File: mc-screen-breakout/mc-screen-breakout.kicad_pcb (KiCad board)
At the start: 4 copper layers, 32 x 20 mm, 28 parts, among them J1 USB_C_Receptacle_PowerOnly_6P, J2 FH28-10S-0.5SH_05_, SW1 NANOT160BP, SW2 NANOT160BP, U1 CMM-3424DT-26165-TR, U2 MDBT50Q-1MV2, Y1 32.768kHz

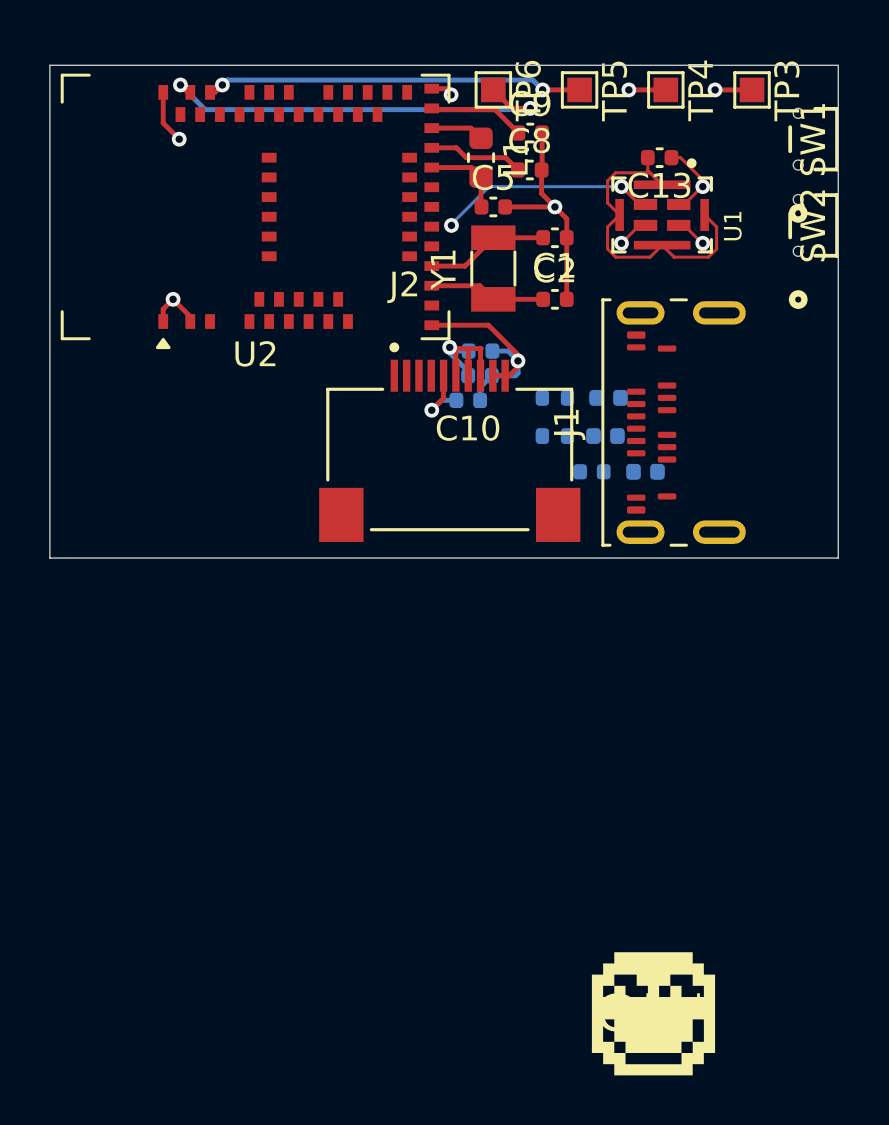
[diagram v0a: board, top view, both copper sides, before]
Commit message: More routing
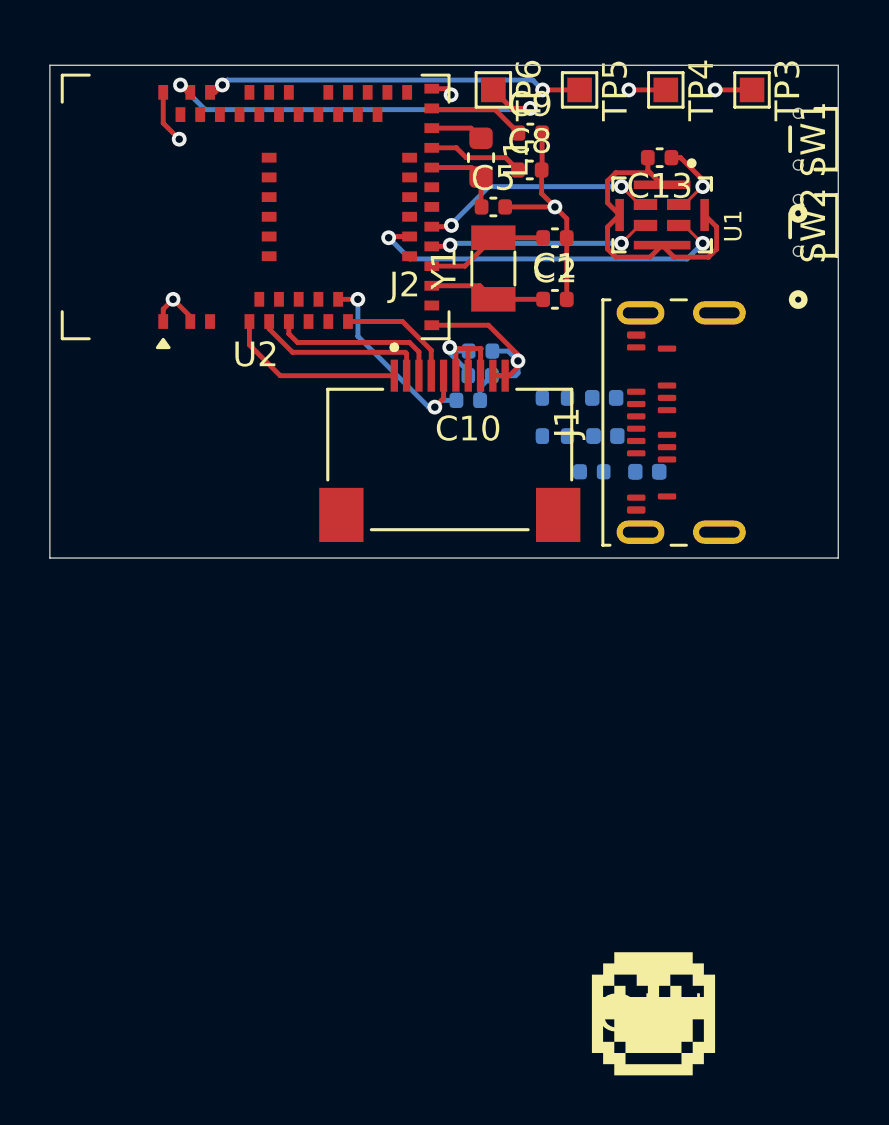
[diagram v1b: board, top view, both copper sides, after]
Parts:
- moved D2 0.17 mm to (58.0, 28.0)
- moved D3 0.08 mm to (59.8, 31.0)
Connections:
- C3 pad 1: +BATT -> Net-(D3-A1)
- D1 pad 2: Net-(D1-A2) -> GND
- D2 pad 2: Net-(D2-A2) -> GND
- D3 pad 2: +BATT -> GND
- R1 pad 1: Net-(D1-A2) -> Net-(D1-A1)
- R2 pad 2: Net-(D2-A2) -> Net-(D2-A1)
- U2 pad 13: unconnected-(U2-P0.28-Pad13) -> LCD_DISP
- U2 pad 14: unconnected-(U2-P0.30-Pad14) -> LCD_EXCOMIN
- U2 pad 16: LCD_DISP -> unconnected-(U2-P0.27-Pad16)
- U2 pad 19: LCD_EXCOMIN -> unconnected-(U2-P0.26-Pad19)
- U2 pad 20: unconnected-(U2-P0.04-Pad20) -> MIC_CLK
- U2 pad 21: unconnected-(U2-P0.05-Pad21) -> MIC_DATA
- U2 pad 22: unconnected-(U2-P0.06-Pad22) -> MIC_SELECT
- U2 pad 4: unconnected-(U2-P1.11-Pad4) -> LCD_SCK
- U2 pad 42: MIC_SELECT -> unconnected-(U2-P0.19-Pad42)
- U2 pad 43: MIC_CLK -> unconnected-(U2-P0.21-Pad43)
- U2 pad 44: MIC_DATA -> unconnected-(U2-P0.20-Pad44)
- U2 pad 45: LCD_SCK -> unconnected-(U2-P0.23-Pad45)
- U2 pad 48: LCD_SI -> unconnected-(U2-P0.24-Pad48)
- U2 pad 49: LCD_CS -> unconnected-(U2-P0.25-Pad49)
- U2 pad 6: unconnected-(U2-P1.13-Pad6) -> LCD_SI
- U2 pad 8: unconnected-(U2-P1.15-Pad8) -> LCD_CS
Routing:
- net MIC_DATA: track 1.28 -> 15.5 mm, vias 1 -> 2
- net MIC_CLK: track 1.28 -> 9.03 mm, vias 1 -> 2
- net LCD_SCK: track 0.00 -> 7.35 mm
- net LCD_SI: track 0.00 -> 7.19 mm
- net LCD_CS: track 0.00 -> 7.05 mm
- net LCD_DISP: track 2.79 -> 9.06 mm, vias 1 -> 2
- net LCD_EXCOMIN: track 0.00 -> 4.90 mm
- net MIC_SELECT: track 8.93 -> 9.75 mm
- net GND: track 39.5 -> 38.8 mm
